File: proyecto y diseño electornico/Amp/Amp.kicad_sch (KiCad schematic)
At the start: 24 parts, among them J1 Cable_PAD, J2 Cable_PAD, J3 Cable_PAD, J4 Cable_PAD, J5 Cable_PAD, J6 Cable_PAD, Q1 BC546, Q2 LND150, U1 TA8200AH

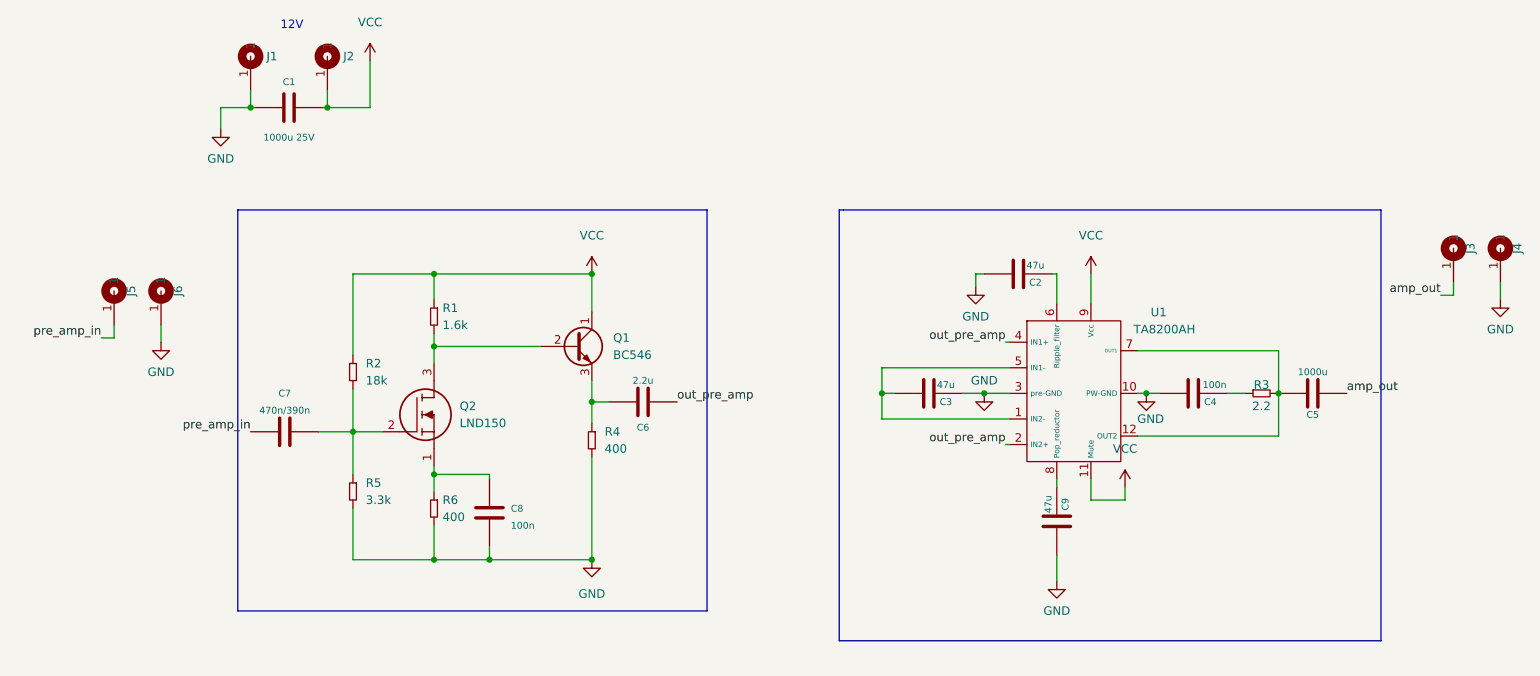
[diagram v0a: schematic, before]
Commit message: 1/11
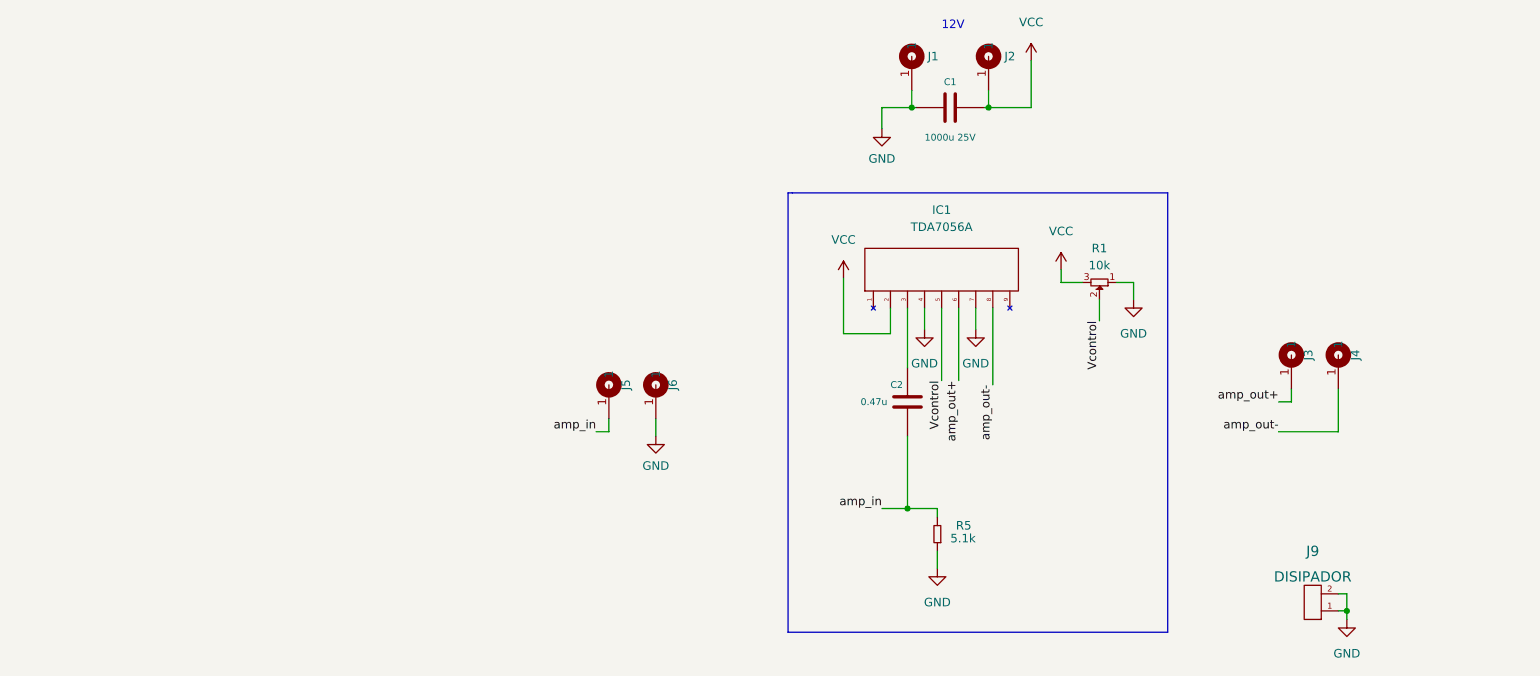
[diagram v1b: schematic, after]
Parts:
- removed C3, C9: 47u, EESTN5:CAP_ELEC_5x11mm, symbol EESTN5:C
- removed C4, C8: 100n, EESTN5:CAP_0.1, symbol EESTN5:C
- removed C5: 1000u, EESTN5:CAP_ELEC_8x11.5mm, symbol EESTN5:C
- removed C6: 2.2u, EESTN5:CAP_ELEC_5x11mm, symbol EESTN5:C
- removed C7: 470n/390n, EESTN5:CAP_0.1, symbol EESTN5:C
- removed Q1: BC546, EESTN5:to92, symbol EESTN5:BC546
- removed Q2: LND150, EESTN5:to92, symbol Macrolib:LND150
- removed R1: 1.6k, EESTN5:RES0.2, symbol EESTN5:R
- removed R2: 18k, EESTN5:RES0.2, symbol EESTN5:R
- removed R3: 2.2, EESTN5:RES0.2, symbol EESTN5:R
- removed R4, R6: 400, EESTN5:RES0.2, symbol EESTN5:R
- removed U1: TA8200AH, MacroLib:hzip12-p-1.78, symbol Macrolib:TA8200AH
- added IC1: TDA7056A, MacroLib:SOT-110, symbol Macrolib:TDA7056A
- added J9: DISIPADOR, MacroLib:Disipador_SOT110-1, symbol EESTN5:HEADER_2
- added R1: 10k, EESTN5:Potenciometro, symbol EESTN5:POT
- C2: value 47u -> 0.47u
- R5: value 3.3k -> 5.1k; footprint EESTN5:RES0.2 -> EESTN5:RES0.3
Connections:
- net GND: now also R5.1, IC1.4 (GND1), IC1.7 (GND2), J9.1, J9.2, R1.1; no longer C2.2, J4.1, R5.2
- net VCC: now also IC1.2 (Vcc), R1.3
- net at C2.1: now also IC1.3 (Vin)
- net amp_out renamed amp_out+
- net amp_out+: now also IC1.6 (OUT+)
- net pre_amp_in renamed amp_in
- net amp_in: now also C2.2, R5.2
- new net Vcontrol: IC1.5 (VC), R1.2
- new net amp_out-: IC1.8 (OUT-), J4.1
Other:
- moved on the sheet: C1, J1, J2, J3, J4, J5, J6
